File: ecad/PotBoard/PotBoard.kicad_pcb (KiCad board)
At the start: 2 copper layers, 35 x 72.8 mm, 38 parts, among them J1 toIOBoard, Q1 2N4401BU, Q2 2N4401BU, U1 RC4558

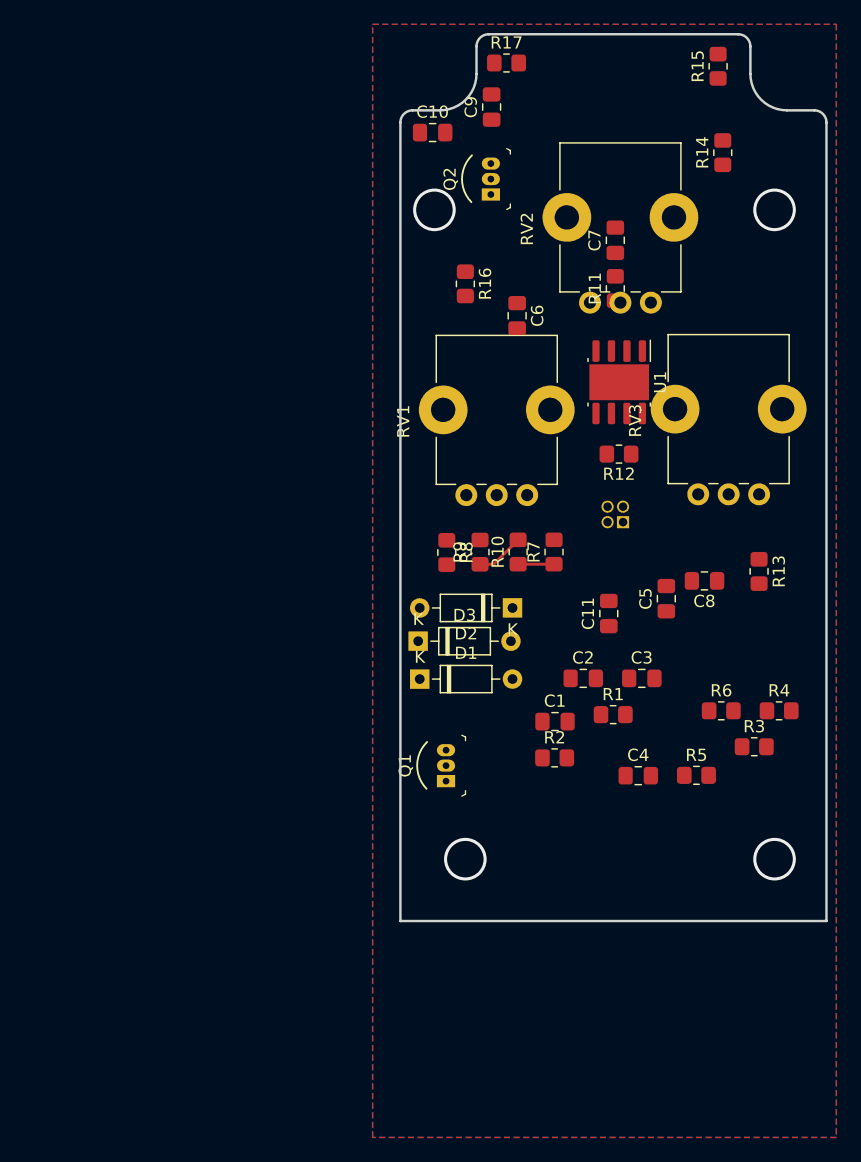
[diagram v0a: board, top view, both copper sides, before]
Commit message: Big commit
Spice Simulations
Finalize ECAD schematic
old MCAD stuff
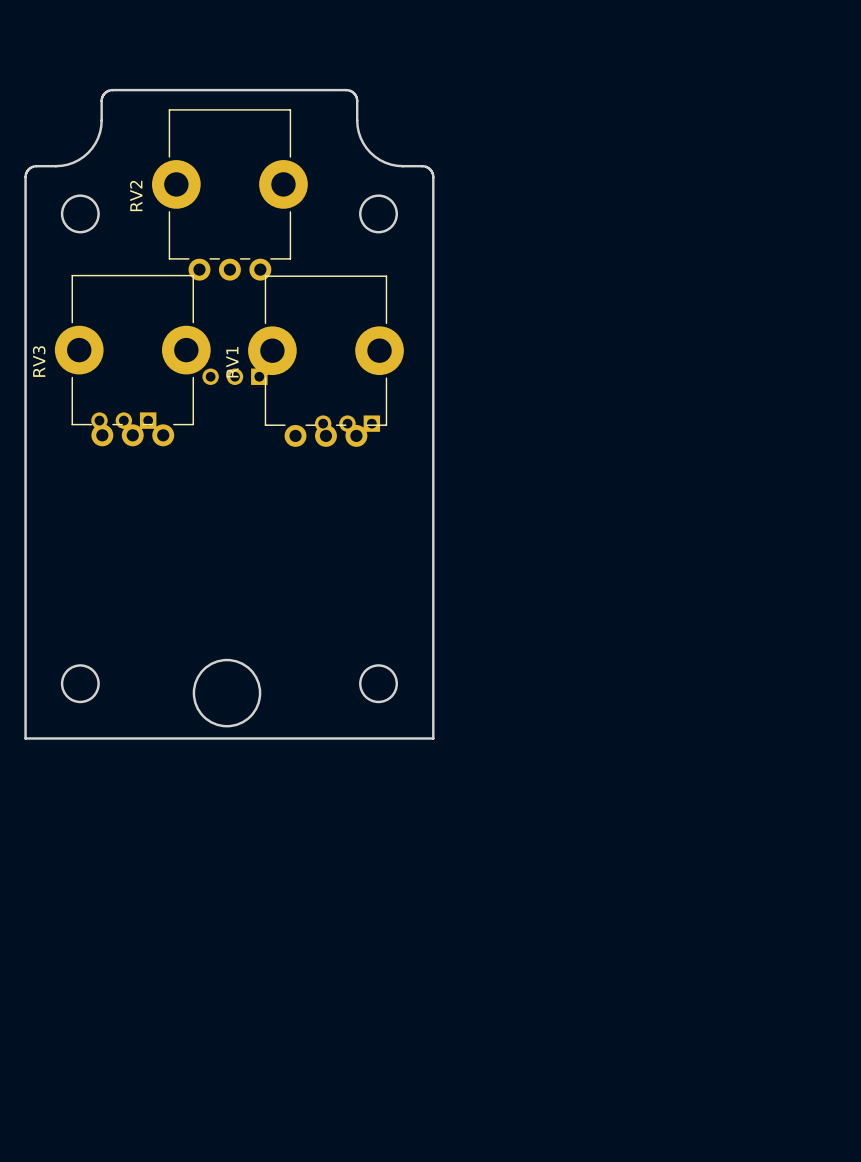
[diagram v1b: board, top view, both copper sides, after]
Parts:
- removed C1: 100u, Capacitor_SMD:C_0805_2012Metric_Pad1.18x1.45mm_HandSolder
- removed C10: CP, Capacitor_SMD:C_0805_2012Metric_Pad1.18x1.45mm_HandSolder
- removed C11: 51p, Capacitor_SMD:C_0805_2012Metric_Pad1.18x1.45mm_HandSolder
- removed C2: 10n, Capacitor_SMD:C_0805_2012Metric_Pad1.18x1.45mm_HandSolder
- removed C3: 47u, Capacitor_SMD:C_0805_2012Metric_Pad1.18x1.45mm_HandSolder
- removed C4: 20n, Capacitor_SMD:C_0805_2012Metric_Pad1.18x1.45mm_HandSolder
- removed C5, C8: 1u, Capacitor_SMD:C_0805_2012Metric_Pad1.18x1.45mm_HandSolder
- removed C6: 0u22, Capacitor_SMD:C_0805_2012Metric_Pad1.18x1.45mm_HandSolder
- removed C7: 220n, Capacitor_SMD:C_0805_2012Metric_Pad1.18x1.45mm_HandSolder
- removed C9: 0u1, Capacitor_SMD:C_0805_2012Metric_Pad1.18x1.45mm_HandSolder
- removed D1, D2, D3: 1N914, Diode_THT:D_DO-35_SOD27_P7.62mm_Horizontal
- removed Q1, Q2: 2N4401BU, digikey-footprints:TO-92-3
- removed R1, R10, R15, R17, R2, R6, R7: 10k, Resistor_SMD:R_0805_2012Metric_Pad1.20x1.40mm_HandSolder
- removed R11: 220, Resistor_SMD:R_0805_2012Metric_Pad1.20x1.40mm_HandSolder
- removed R12, R13, R4, R9: 1k, Resistor_SMD:R_0805_2012Metric_Pad1.20x1.40mm_HandSolder
- removed R14, R5: 501k, Resistor_SMD:R_0805_2012Metric_Pad1.20x1.40mm_HandSolder
- removed R16: 100, Resistor_SMD:R_0805_2012Metric_Pad1.20x1.40mm_HandSolder
- removed R3: 1M5, Resistor_SMD:R_0805_2012Metric_Pad1.20x1.40mm_HandSolder
- removed R8: 51k, Resistor_SMD:R_0805_2012Metric_Pad1.20x1.40mm_HandSolder
- removed U1: RC4558, Package_SO:Texas_R-PDSO-G8_EP2.95x4.9mm_Mask2.4x3.1mm
- added J2: TonePot, Connector_PinSocket_2.00mm:PinSocket_1x03_P2.00mm_Vertical, B.Cu at (102.5, 79.8)
- added J3: VolumePot, Connector_PinSocket_2.00mm:PinSocket_1x03_P2.00mm_Vertical, B.Cu at (93.3, 83.3)
- J1: value toIOBoard -> DrivePot; footprint Connector_PinSocket_1.27mm:PinSocket_2x02_P1.27mm_Vertical -> Connector_PinSocket_2.00mm:PinSocket_1x03_P2.00mm_Vertical
- RV2: value 20k -> 20kb
- moved RV3 49.2 mm to (94.6, 84.6)
- moved RV2 32.2 mm to (102.5, 71.0)
- moved J1 22.2 mm to (111.7, 83.6), turned to 90 degrees
- moved RV1 14.8 mm to (110.4, 84.6)
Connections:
- J1 pad 1: +9V -> Net-(J1-Pad1)
- J1 pad 2: SIG_IN -> Net-(J1-Pad2)
- J1 pad 3: GND -> Net-(J1-Pad3)
- RV1 pad 1: Net-(R8-Pad1) -> Net-(J1-Pad1)
- RV1 pad 2: Net-(C11-Pad1) -> Net-(J1-Pad2)
- RV1 pad 3: Net-(RV1-Pad3) -> Net-(J1-Pad3)
- RV2 pad 1: DRIVE_OUT -> Net-(J2-Pad1)
- RV3 pad 2: VCC -> Net-(J3-Pad2)
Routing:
- net DRIVE_OUT: track 3.96 -> 0.00 mm
- net VCC: track 2.95 -> 0.00 mm
- net Net-(Q2-Pad1): vias 1 -> 0
- net (no net): vias 3 -> 0
- removed copper zone on F.Cu, net +9V
- removed copper zone on B.Cu, net GND
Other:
- board size 35 x 72.8 mm -> 33.5 x 53.3 mm
